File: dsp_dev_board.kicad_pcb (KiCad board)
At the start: 2 copper layers, 100 x 60.3 mm, 74 parts, among them J1 aux_mcu_power, J10 DX07S016JA1R1500, J11 Conn_02x08_Odd_Even, J2 audio_in, J3 audio_out, J4 9v_jack, J5 input_jack, J6 output_jack, J7 PD8-15 (digital), J8 PA0-7 (analog), J9 debug, U1 TL072, U2 AMS1117-3.3, U3 STM32F407VETx, U4 WM8731SEDS, Y1 8Mhz

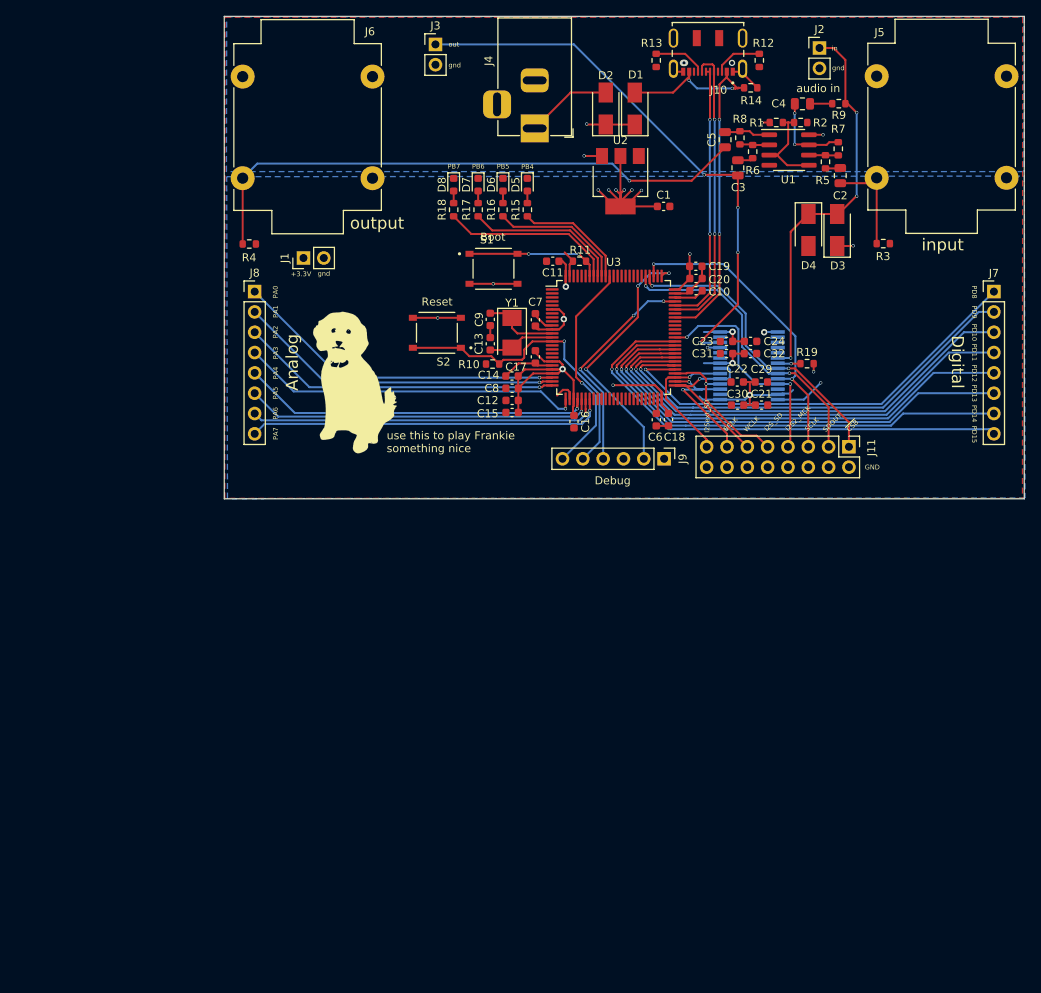
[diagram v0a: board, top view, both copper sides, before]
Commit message: 4 layer progress
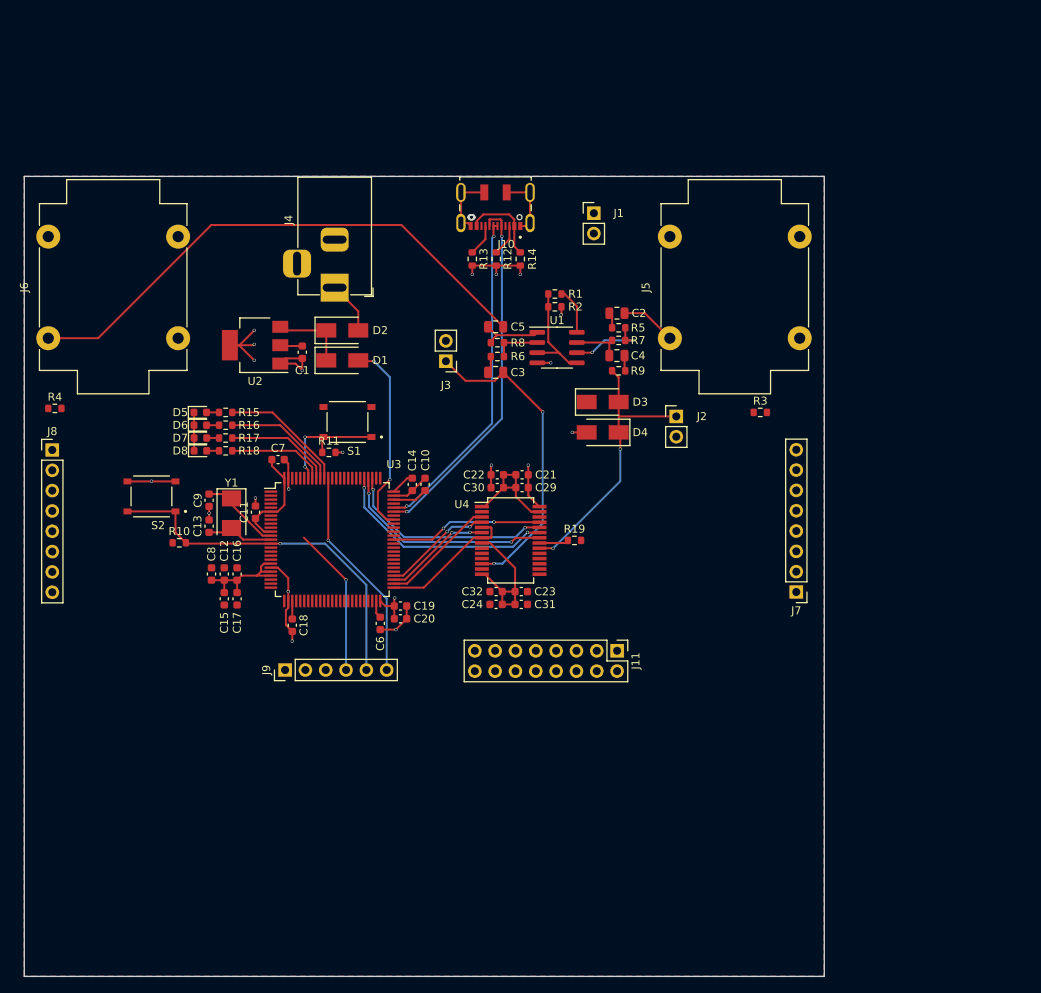
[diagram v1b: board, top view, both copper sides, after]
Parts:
- removed G***: LOGO, frankie:frankie
- J10: footprint USB_C:JAE_DX07S016JA1R1500 -> DX07S016JA1R1500:JAE_DX07S016JA1R1500
- U4: moved to F.Cu
- moved C20 56.3 mm to (137.0, 95.3)
- moved C19 56.3 mm to (137.0, 93.7)
- moved J9 54.2 mm to (122.6, 101.7), turned to 90 degrees
- moved C18 53.6 mm to (123.5, 96.1)
- moved U2 50.1 mm to (118.8, 61.1), turned to 180 degrees
- moved D5 49.8 mm to (112.0, 69.5), turned to 0 degrees
- moved J2 49.4 mm to (171.5, 70.0)
- moved C1 48.7 mm to (124.8, 62.0), turned to 270 degrees
- moved C11 48.6 mm to (118.9, 82.0), turned to 90 degrees
- moved D6 48.3 mm to (112.0, 71.1), turned to 0 degrees
- moved D1 48.2 mm to (129.8, 63.0), turned to 0 degrees
- moved C17 48.0 mm to (116.6, 92.8)
- moved D7 47.0 mm to (112.0, 72.7), turned to 0 degrees
- moved C16 46.2 mm to (116.6, 89.7), turned to 90 degrees
- moved D8 45.9 mm to (112.0, 74.3), turned to 0 degrees
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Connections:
- R10 pad 1: /MCU/NRST -> 3.3V
- R10 pad 2: GND -> /MCU/NRST
- S2 pad C: 3.3V -> GND
- S2 pad D: 3.3V -> GND
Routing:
- net Net-(J7-Pad8): track 61.0 -> 0.00 mm, vias 1 -> 0
- net Net-(J7-Pad7): track 59.7 -> 0.00 mm, vias 1 -> 0
- net Net-(J7-Pad6): track 58.9 -> 0.00 mm, vias 1 -> 0
- net Net-(J7-Pad5): track 58.2 -> 0.00 mm, vias 1 -> 0
- net Net-(J7-Pad4): track 57.4 -> 0.00 mm, vias 1 -> 0
- net Net-(J7-Pad3): track 56.6 -> 0.00 mm, vias 1 -> 0
- net Net-(J7-Pad2): track 56.2 -> 0.00 mm, vias 1 -> 0
- net Net-(J7-Pad1): track 54.8 -> 0.00 mm, vias 1 -> 0
- net GND: track 40.2 -> 86.2 mm, vias 3 -> 17
- net 3.3V: track 130.6 -> 84.9 mm, vias 18 -> 4
- net Net-(J8-Pad8): track 45.0 -> 0.00 mm, vias 1 -> 0
- net Net-(J8-Pad5): track 44.2 -> 0.00 mm, vias 1 -> 0
- net Net-(J8-Pad7): track 44.0 -> 0.00 mm, vias 1 -> 0
- net Net-(J8-Pad6): track 43.9 -> 0.00 mm, vias 1 -> 0
- net Net-(J8-Pad4): track 43.0 -> 0.00 mm, vias 1 -> 0
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- added copper zone on F.Cu, net 3.3V
- added copper zone on In1.Cu, net GND
- added copper zone on In2.Cu, net GND
- removed copper zone on B.Cu, net 9V
- removed copper zone on F.Cu, net GND
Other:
- board size 100 x 60.3 mm -> 100 x 100 mm
- copper layers 2 -> 4
- board text removed: "+3.3V"
- board text removed: "Analog"
- board text removed: "BCLK"
- board text removed: "Boot"
- board text removed: "DSP dev board v1 by Eric Wood"
- board text removed: "Debug"
- board text removed: "Digital"
- board text removed: "GND"
- board text removed: "I2S2_MCK"
- board text removed: "I2S_SD"
- board text removed: "I2Sext_SD"
- board text removed: "PA0"
- board text removed: "PA1"
- board text removed: "PA2"
- board text removed: "PA3"
- board text removed: "PA4"
- board text removed: "PA5"
- board text removed: "PA6"
- board text removed: "PA7"
- board text removed: "PB4"
- board text removed: "PB5"
- board text removed: "PB6"
- board text removed: "PB7"
- board text removed: "PD10"
- board text removed: "PD11"
- board text removed: "PD12"
- board text removed: "PD13"
- board text removed: "PD14"
- board text removed: "PD15"
- board text removed: "PD8"
- board text removed: "PD9"
- board text removed: "Reset"
- board text removed: "SCLK"
- board text removed: "SDOUT"
- board text removed: "WCLK"
- board text removed: "audio in"
- board text removed: "gnd"
- board text removed: "in"
- board text removed: "input"
- board text removed: "out"
- board text removed: "output"
- board text removed: "use this to play Frankie something nice"
- board text removed: "~CSB"
